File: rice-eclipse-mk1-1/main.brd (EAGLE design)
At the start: 110.2 x 91.2 mm, 136 parts, among them IC1 LMV321LICTRT, IC2 LMV321LICTRT, IC3 LMV321LICTRT, IC4 LMV321LICTRT, IC5 UA78M, IC6 LMV321LICTRT, IC7 LMV321LICTRT, IC8 LMV321LICTRT, IC9 LMV321LICTRT, U1 LM1084ISX-5.0/NOPB, U2 THS4531IDRD8-M, U3 THS4531IDRD8-M, U4 THS4531IDRD8-M, U5 THS4531IDRD8-M, U6 1101M2S3CQE2

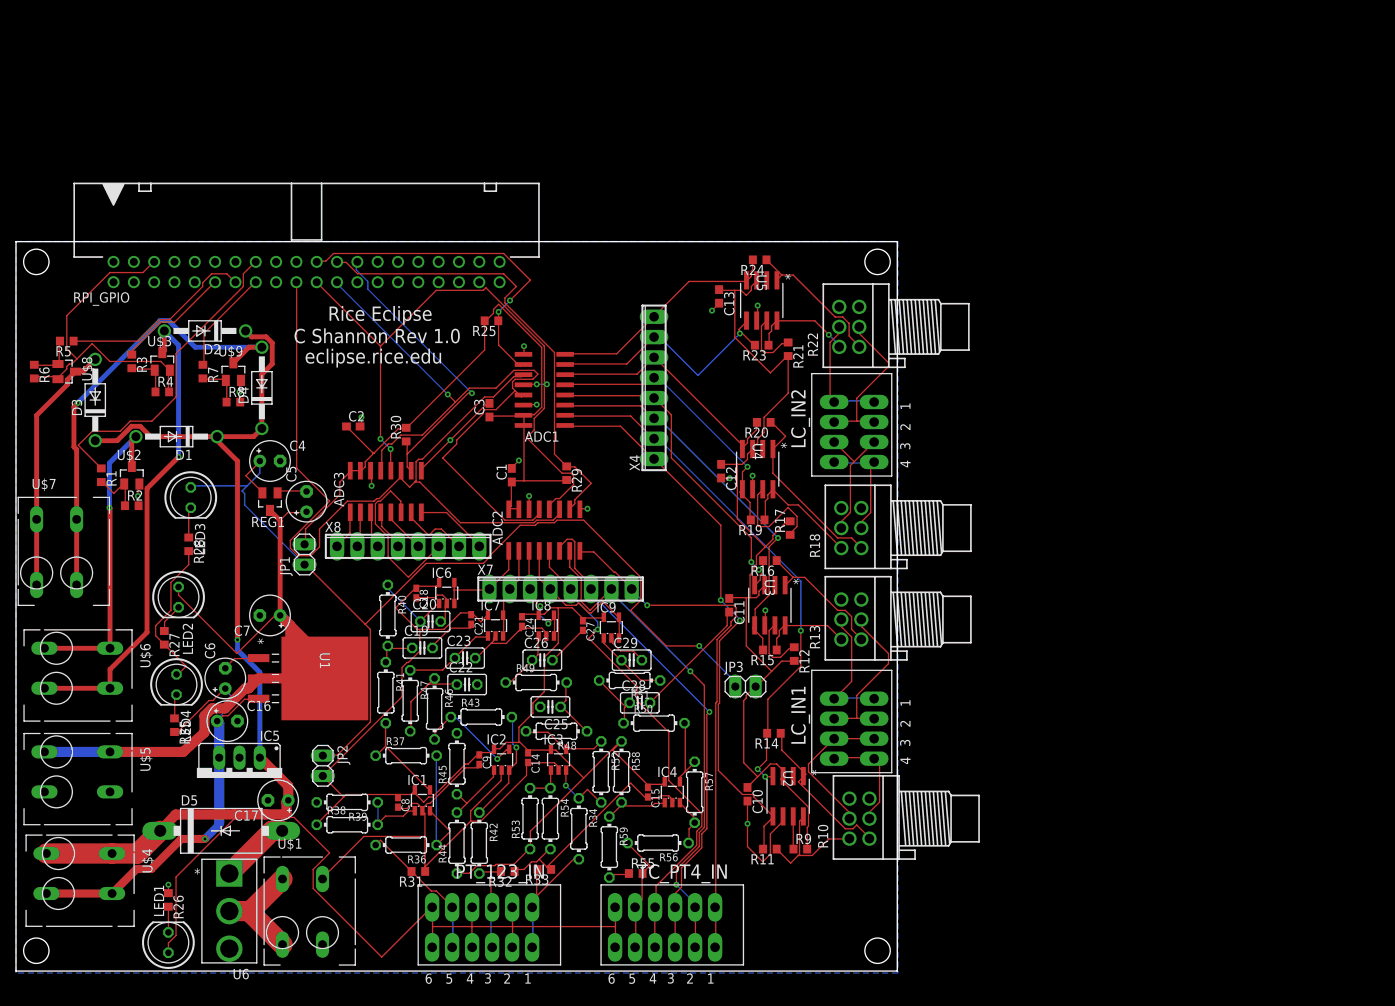
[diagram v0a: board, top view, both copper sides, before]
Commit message: Fixed board files maybe.
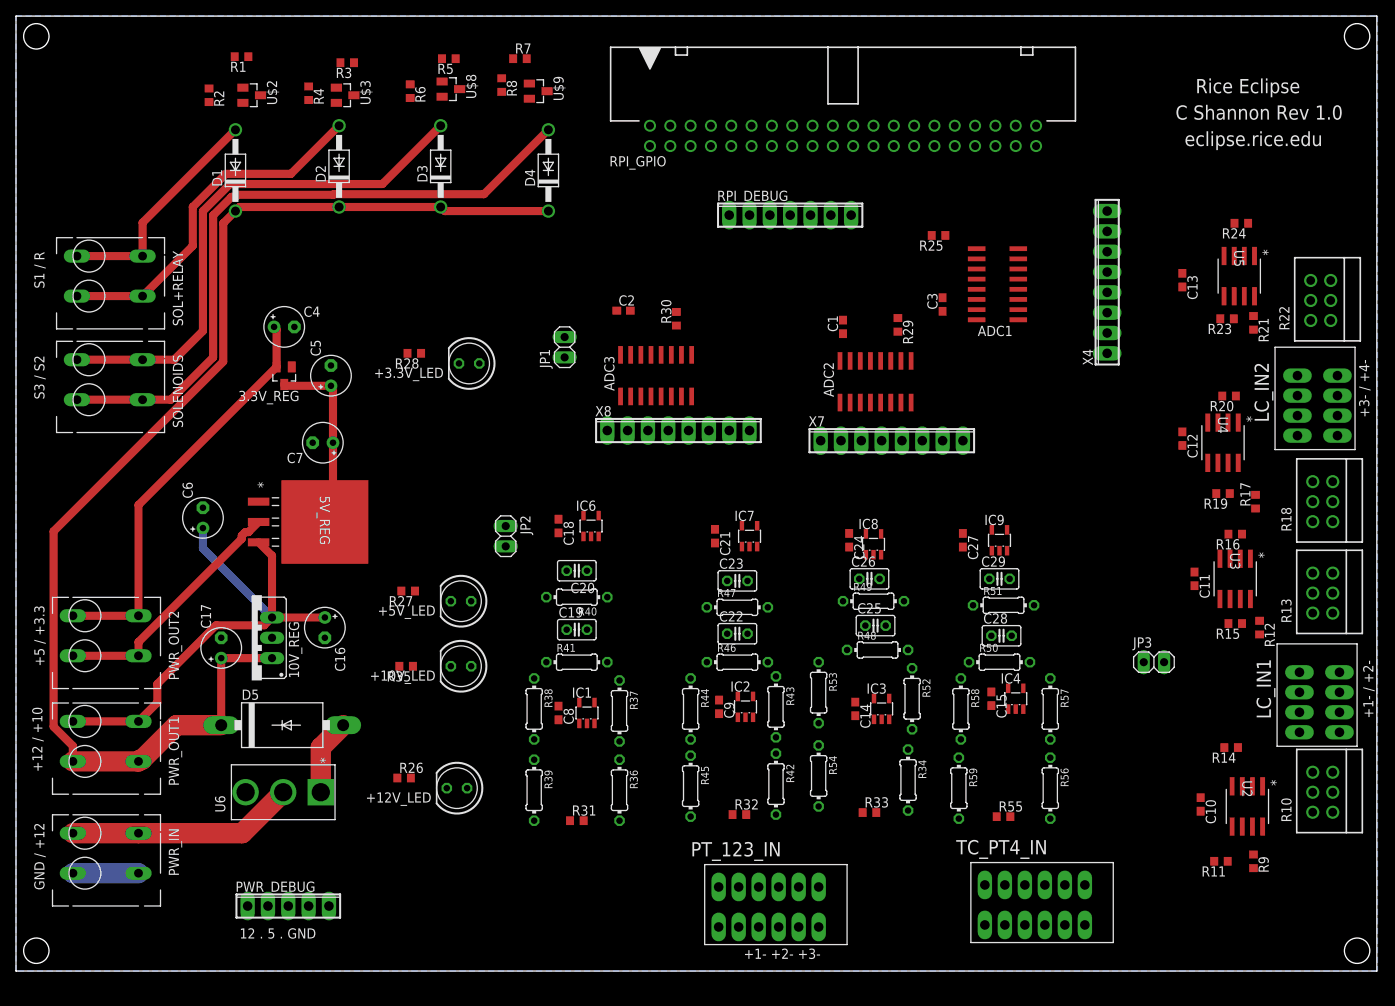
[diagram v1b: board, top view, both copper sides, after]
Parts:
- removed IC5: UA78M, texas-extra:TO220S
- removed LED1, LED2, LED3, LED4: (no value), led:LED5MM
- removed REG1: AP2210N-3.3TRG1, diodes-extra:SOT23
- removed U$1, U$4, U$5, U$6, U$7: 1991095, con-phoenix-500-extra:1991095
- removed U1: LM1084ISX-5.0/NOPB, texas-extra:TS3B
- added +10V_LED, +12V_LED, +3.3V_LED, +5V_LED: (no value), led:LED5MM
- added 10V_REG: UA78M, texas-extra:TO220S
- added 3.3V_REG: AP2210N-3.3TRG1, diodes-extra:SOT23
- added 5V_REG: LM1084ISX-5.0/NOPB, texas-extra:TS3B
- added PWR_DEBUG: (no value), con-phoenix-254:5POL254
- added PWR_IN, PWR_OUT1, PWR_OUT2, SOL+RELAY, SOLENOIDS: 1991095, con-phoenix-500-extra:1991095
- added RPI_DEBUG: (no value), con-phoenix-254:7POL254
- C14, C15, C18, C21, C24, C27, C8, C9: value 10nF -> 0.1UF; device rcl:C0402K -> rcl:C0603
- moved RPI_GPIO 69.2 mm to (103.4, 104.4)
- moved R24 60.4 mm to (153.2, 93.5)
- moved U5 59.8 mm to (152.9, 86.9)
- moved U$8 59.6 mm to (54.4, 110.2)
- moved R5 59.4 mm to (54.1, 114.0)
- moved R13 59.0 mm to (164.6, 47.2)
- moved R18 59.0 mm to (164.6, 58.7)
- moved R22 59.0 mm to (164.3, 83.8)
- moved R6 58.6 mm to (49.3, 110.0)
- moved LC_IN1 58.3 mm to (157.7, 40.9)
- moved R12 58.3 mm to (155.4, 42.9)
- moved R15 58.3 mm to (152.4, 43.4)
- moved R16 58.3 mm to (152.4, 54.6)
- moved R19 58.3 mm to (150.9, 59.7)
- moved R20 58.3 mm to (151.6, 71.9)
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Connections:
- net +10V: now also 10V_REG.3, 5V_REG.3, PWR_DEBUG.2, PWR_OUT1.A1, PWR_OUT1.B1; no longer IC5.3, U$4.A2, U$4.B2, U1.3
- net +12V: now also +12V_LED.A, 10V_REG.1, PWR_DEBUG.1, PWR_OUT1.A2, PWR_OUT1.B2; no longer IC5.1, LED1.A, U$4.A1, U$4.B1
- net +12V_DEBUG: now also PWR_IN.A1, PWR_IN.B1; no longer U$1.A1, U$1.B1
- net +3V3: now also +3.3V_LED.A, 3.3V_REG.2, PWR_DEBUG.4, PWR_OUT2.A1, PWR_OUT2.B1; no longer LED3.A, REG1.2
- net +5V: now also +5V_LED.A, 3.3V_REG.3, 5V_REG.2, 5V_REG.4, PWR_DEBUG.3, PWR_OUT2.A2, PWR_OUT2.B2; no longer LED2.A, REG1.3, U$5.A1, U$5.B1, U1.2, U1.4
- net ADC1_CS: now also RPI_DEBUG.4
- net ADC2_CS: now also RPI_DEBUG.3
- net ADC3_CS: now also RPI_DEBUG.2
- net GND: now also +10V_LED.K, 10V_REG.2, 3.3V_REG.1, 5V_REG.1, PWR_DEBUG.5, PWR_IN.A2, PWR_IN.B2, RPI_DEBUG.1; no longer IC5.2, LED4.A, REG1.1, U$1.A2, U$1.B2, U$5.A2, U$5.B2, U1.1
- net MISO: now also RPI_DEBUG.6
- net MOSI: now also RPI_DEBUG.5
- net N$1: now also +12V_LED.K; no longer LED1.K
- net N$2: now also +5V_LED.K; no longer LED2.K
- net N$3: now also +3.3V_LED.K; no longer LED3.K
- net N$9: now also +10V_LED.A; no longer LED4.K
- net RELAY_NEGATIVE: now also SOL+RELAY.A1, SOL+RELAY.B1; no longer U$6.A1, U$6.B1
- net SCLK: now also RPI_DEBUG.7
- net SOLENOID_1_NEGATIVE: now also SOL+RELAY.A2, SOL+RELAY.B2; no longer U$6.A2, U$6.B2
- net SOLENOID_2_NEGATIVE: now also SOLENOIDS.A1, SOLENOIDS.B1; no longer U$7.A1, U$7.B1
- net SOLENOID_3_NEGATIVE: now also SOLENOIDS.A2, SOLENOIDS.B2; no longer U$7.A2, U$7.B2
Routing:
- net GND: track 276.6 -> 8.20 mm, vias 17 -> 0
- net +3V3_PT: track 161.6 -> 0.00 mm
- net +3V3_LC: track 116.3 -> 0.00 mm
- net MOSI: track 102.6 -> 0.00 mm
- net +3V3_ADC: track 88.8 -> 0.00 mm
- net MISO: track 83.1 -> 0.00 mm, vias 4 -> 0
- net SCLK: track 83.1 -> 0.00 mm, vias 1 -> 0
- net +3V3: track 125.7 -> 51.6 mm, vias 1 -> 0
- net ADC1_A0: track 71.4 -> 0.00 mm, vias 2 -> 0
- net ADC2_A7: track 66.3 -> 0.00 mm, vias 1 -> 0
- net ADC1_A1: track 66.2 -> 0.00 mm, vias 3 -> 0
- net +12V: track 218.4 -> 153.9 mm, vias 1 -> 0
- net ADC2_A6: track 64.3 -> 0.00 mm, vias 2 -> 0
- net ADC2_A5: track 62.7 -> 0.00 mm, vias 1 -> 0
- net ADC2_A4: track 60.8 -> 0.00 mm, vias 1 -> 0
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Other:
- board size 110.2 x 91.2 mm -> 170.1 x 119.4 mm
